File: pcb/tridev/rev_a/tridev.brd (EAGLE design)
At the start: 102.7 x 72.5 mm, 41 parts, among them J15 MICRO_USB_B_HIROSE_ZX62R-B-5P, J3 TC2030-JLINK-L, J4 TC2030-JLINK-L, U1 NRF51822QF, U2 TRIPOINT-BREAKOUT, U4 MAX8887EZK33+T, X1 EPSON-FA-128

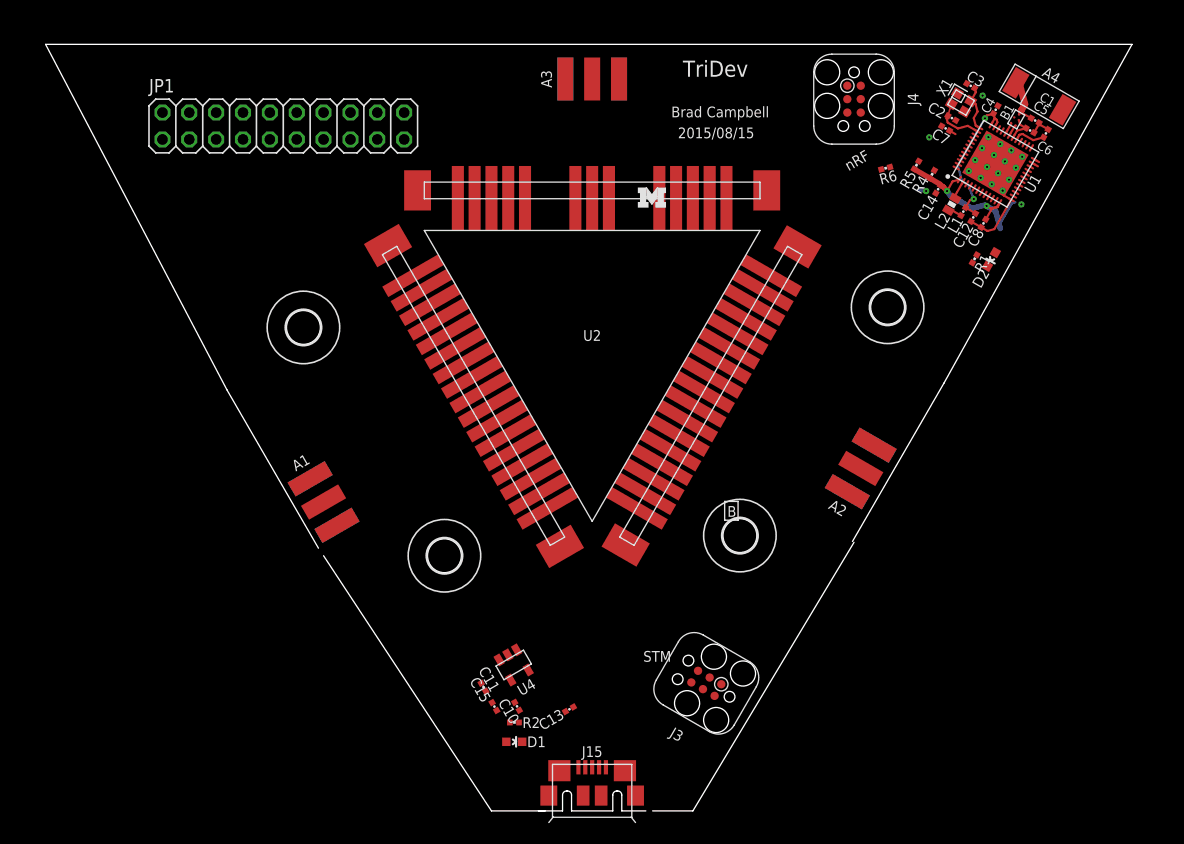
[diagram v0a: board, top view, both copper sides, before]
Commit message: breakout basically done
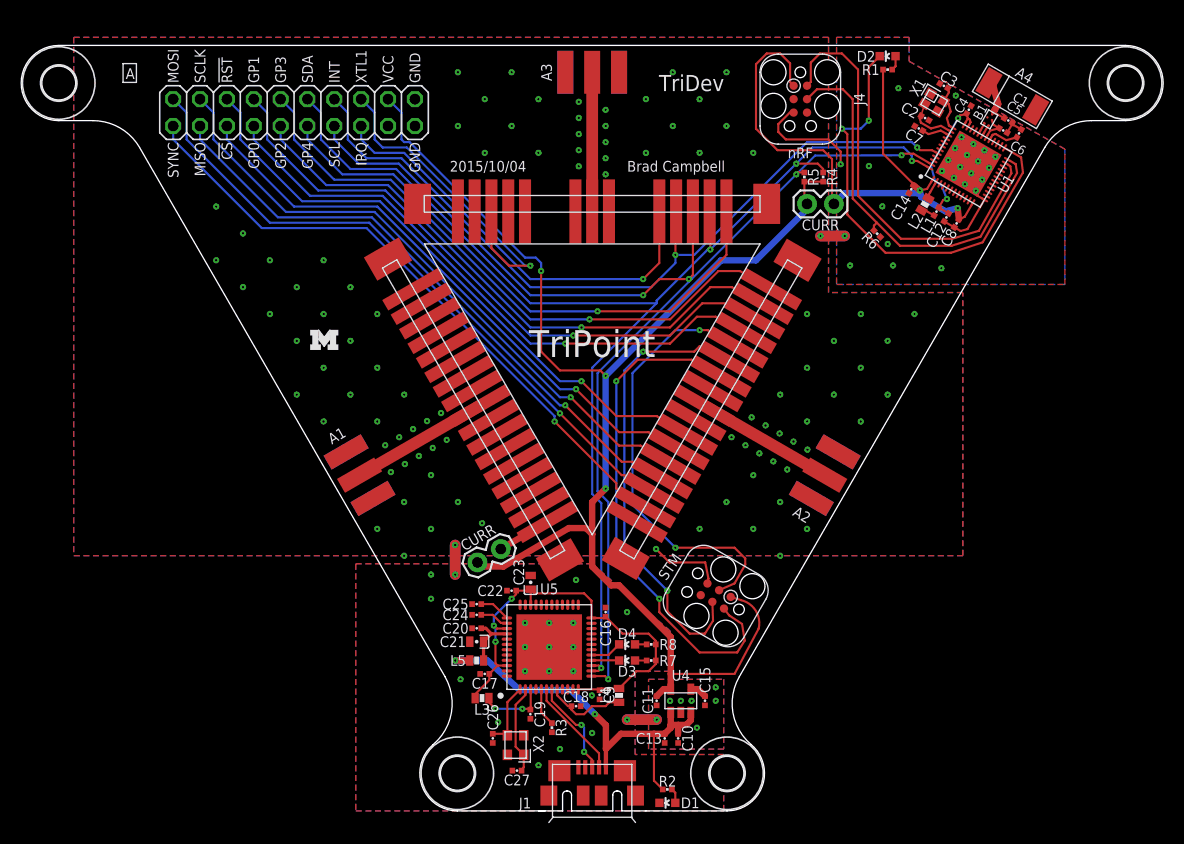
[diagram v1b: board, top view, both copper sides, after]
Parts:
- removed H5, H6, H7, H8: MOUNT-HOLE3.2, holes:3,2
- removed JP1: (no value), pinhead:2X10
- added C16, C17, C18, C19, C20, C22, C24, C25, C9: 0.1uF, passives:0402_CAP
- added C21, C23: 4.7uF, passives:CAP0603
- added C26, C27: 18pF, passives:0402_CAP
- added D3: RED, SparkFun-LED:LED-0603
- added D4: BLUE, SparkFun-LED:LED-0603
- added H1, H2, H3, H4: MOUNT-HOLE3.2, holes:3,2
- added J2: (no value), pinhead:2X10
- added J5, J6: (no value), SparkFun-Passives:1X02
- added L3, L4, L5: FERRITE_BEAD, passives:0603_CAP
- added R3: 12k 1%, passives:0402_RES
- added R7, R8: 1k, passives:0402_RES
- added U5: FT232HQ, chips:QFN-48-8MM
- added X2: TXC-8Z-12MHZ, crystals:TXC-8Z
- moved LOGO1 33.8 mm to (-26.7, -0.86)
- moved D2 21.6 mm to (27.9, 26.9), turned to 90 degrees
- moved C15 19.9 mm to (10.7, -34.0), turned to 270 degrees
- moved R1 19.7 mm to (27.9, 25.7), turned to 180 degrees
- moved C11 16.4 mm to (6.10, -34.0), turned to 270 degrees
- moved U4 16.2 mm to (8.38, -34.0), turned to 0 degrees
- moved R2 15.8 mm to (7.11, -42.4), turned to 180 degrees
- moved D1 15.6 mm to (7.11, -43.7), turned to 90 degrees
- moved C10 15.5 mm to (8.13, -37.6), turned to 270 degrees
- moved R5 10.7 mm to (20.1, 15.5), turned to 270 degrees
- moved R4 10.3 mm to (21.8, 15.5), turned to 270 degrees
- moved C13 9.42 mm to (6.86, -37.6), turned to 270 degrees
- moved J3 8.30 mm to (11.7, -24.1)
- moved R6 6.25 mm to (26.9, 10.1), turned to 135 degrees
- moved J4 5.08 mm to (19.7, 22.9)
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- renumbered J15 to J1
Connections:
- removed net DW_INT: U1.44, U2.38
- new net !DW_CS: J2.5, U2.23
- new net !DW_RST: J2.6, U2.24
- new net DW_CLK: J2.4, U2.22
- new net DW_IRQ: J2.15, U2.39
- new net DW_MISO: J2.3, U2.21
- new net DW_MOSI: J2.2, U2.20
- new net DW_SYNC: J2.1, U2.19
- new net DW_XTAL1: J2.16, U2.49
- new net N$12: C20.1, C21.POS, L5.2, U5.40
- new net N$13: C24.1, U5.38
- new net N$14: C26.1, U5.1, X2.3
- new net N$16: C27.1, U5.2, X2.1
- new net N$21: C25.1, U5.37
- new net N$22: R3.2, U5.5
- new net N$23: J5.2, U2.17
- new net N$24: D3.A, R7.1
- new net N$25: D4.A, R8.1
- new net N$26: D4.C, U5.17
- new net N$38: J2.17
- new net N$5: D3.C, U5.16
- new net NRF_VCC: C14.1, C8.1, J4.1, J6.2, R1.2, U1.1, U1.12
- new net TP_GPIO0: J2.7, U2.31
- new net TP_GPIO1: J2.8, U2.32
- new net TP_GPIO2: J2.9, U2.33
- new net TP_GPIO3: J2.10, U2.34
- new net TP_GPIO4: J2.11, U2.35
- new net TP_INT: J2.14, U1.44, U2.38
- new net USB_D+: J1.3, U5.7
- new net USB_D-: J1.2, U5.6
- new net VCC3V3: C16.1, C17.1, C22.1, C23.POS, C9.1, L3.2, L4.2, R7.2, R8.2, U5.12, U5.24, U5.34, U5.39, U5.46
- new net VPHY: C19.1, L3.1, U5.3
- new net VPLL: C18.1, L4.1, U5.8
- net GND: now also C16.2, C17.2, C18.2, C19.2, C20.2, C21.NEG, C22.2, C23.NEG, C24.2, C25.2, C26.2, C27.2, C9.2, J2.19, J2.20, R3.1, U5.10, U5.11, U5.22, U5.23, U5.35, U5.36, U5.4, U5.41, U5.42, U5.47, U5.48, U5.9, U5.PAD, X2.2, X2.4
- net I2C_SCL: now also J2.13, U5.13
- net I2C_SDA: now also J2.12, U5.14, U5.15
- net N$1: now also A1.ANT
- net N$2: now also A2.ANT
- net N$3: now also A3.ANT
- net VCC: now also J2.18, J5.1, J6.1; no longer C14.1, C8.1, J4.1, R1.2, U1.1, U1.12, U2.17
- net VUSB: now also L5.1
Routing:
- net I2C_SDA: track 0.00 -> 121.7 mm, vias 0 -> 4
- net I2C_SCL: track 0.00 -> 120.8 mm, vias 0 -> 5
- net VCC: track 18.6 -> 130.5 mm, vias 2 -> 3
- net TP_INT: track 0.00 -> 76.6 mm, vias 0 -> 2
- net DW_MOSI: track 0.00 -> 62.1 mm, vias 0 -> 1
- net DW_SYNC: track 0.00 -> 60.7 mm, vias 0 -> 1
- net DW_CLK: track 0.00 -> 60.0 mm, vias 0 -> 1
- net TP_GPIO1: track 0.00 -> 59.7 mm, vias 0 -> 1
- net TP_GPIO3: track 0.00 -> 58.9 mm, vias 0 -> 1
- net DW_MISO: track 0.00 -> 58.0 mm, vias 0 -> 1
- net !DW_RST: track 0.00 -> 57.9 mm, vias 0 -> 1
- net TP_GPIO0: track 0.00 -> 57.2 mm, vias 0 -> 1
- net NRF_VCC: track 0.00 -> 56.8 mm, vias 0 -> 2
- net TP_GPIO2: track 0.00 -> 56.2 mm, vias 0 -> 1
- net !DW_CS: track 0.00 -> 55.9 mm, vias 0 -> 1
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- added copper zone on layer 1, net GND
- added copper zone on layer 16, net GND
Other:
- board size 102.7 x 72.5 mm -> 108 x 72.4 mm
- board text added: "!CS"
- board text added: "!RST"
- board text added: "2015/10/04"
- board text added: "A"
- board text added: "CURR"
- board text added: "GND"
- board text added: "GP0"
- board text added: "GP1"
- board text added: "GP2"
- board text added: "GP3"
- board text added: "GP4"
- board text added: "INT"
- board text added: "IRQ"
- board text added: "MISO"
- board text added: "MOSI"
- board text added: "SCL"
- board text added: "SCLK"
- board text added: "SDA"
- board text added: "SYNC"
- board text added: "TriPoint"
- board text added: "VCC"
- board text added: "XTL1"
- board text removed: "2015/08/15"
